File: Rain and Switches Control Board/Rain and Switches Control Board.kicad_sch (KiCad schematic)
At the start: 35 parts, among them J1 Conn_01x06_MountingPin, J2 Screw_Terminal_01x02, J3 Conn_01x02, J4 8P8C, J5 Conn_01x02, J6 Conn_01x02, J7 Conn_01x02, J8 Conn_01x02, J9 RJ45, Q1 NPN, Q2 NPN, Q3 NPN, Q4 NPN, Q5 NPN, U2 OKI-78SR

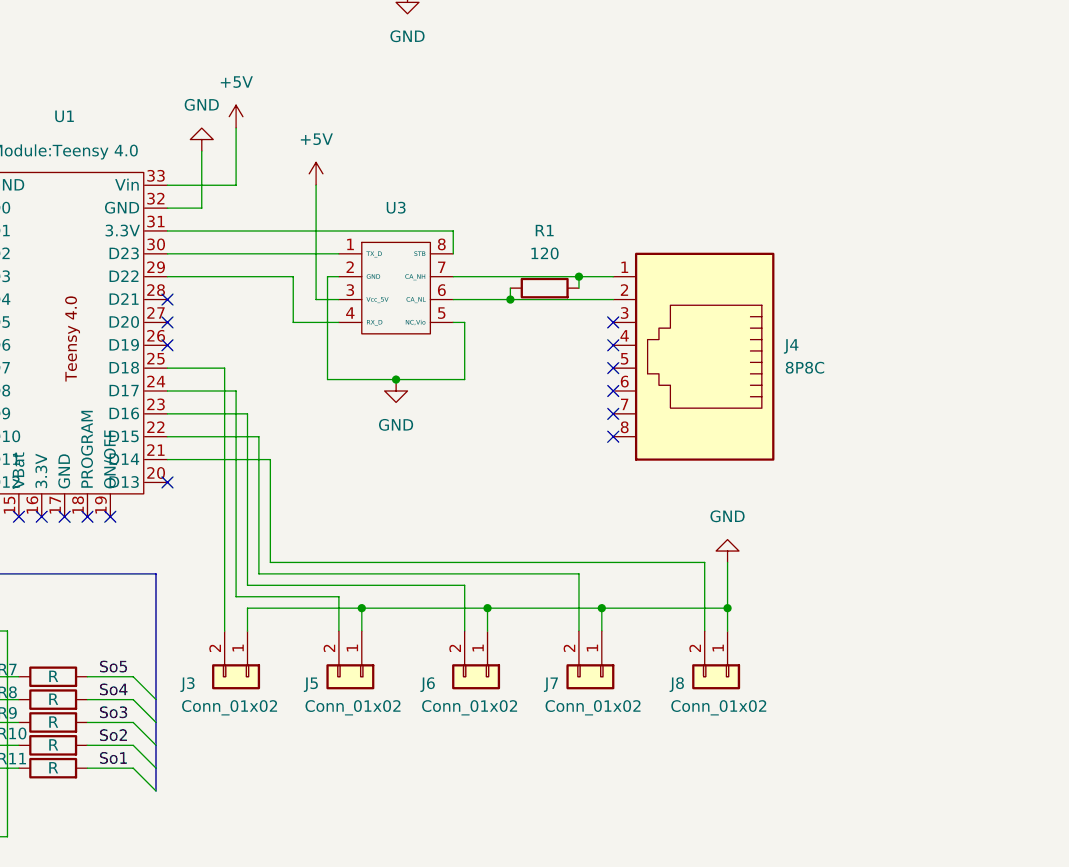
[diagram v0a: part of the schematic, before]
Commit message: Rev. 3
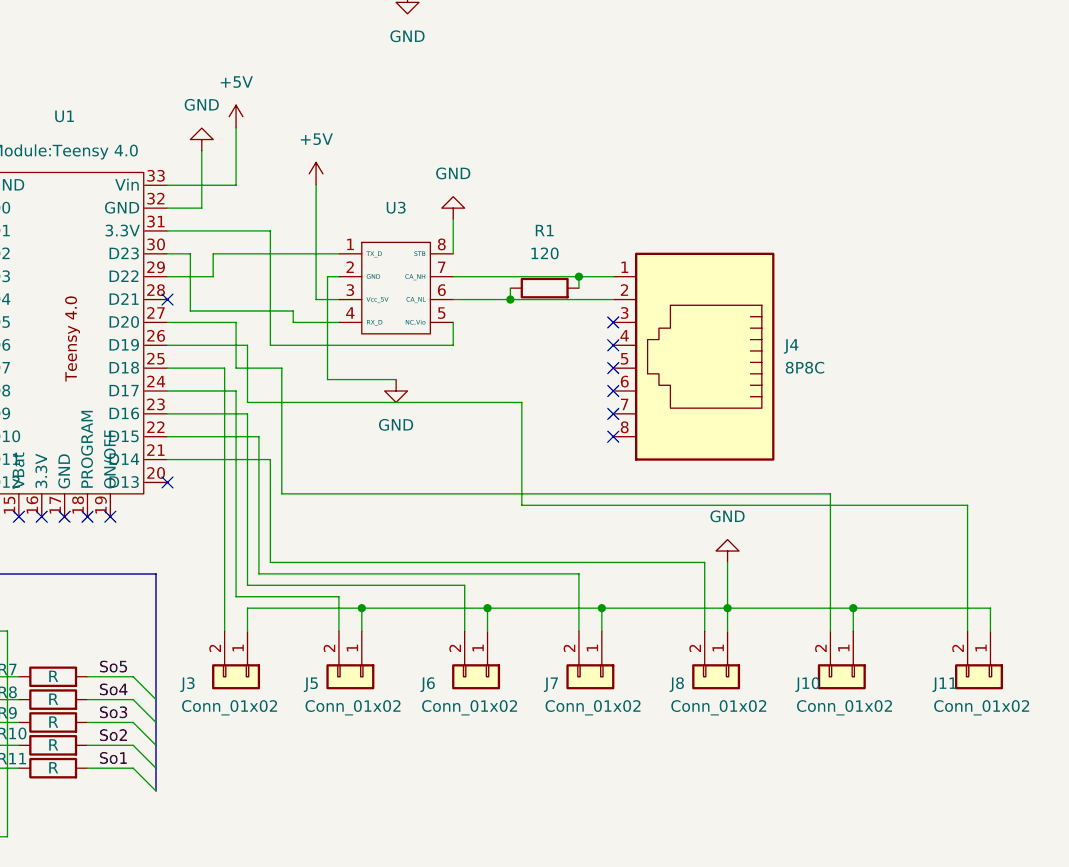
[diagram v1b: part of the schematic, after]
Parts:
- added J10, J11: Conn_01x02, TerminalBlock:TerminalBlock_Altech_AK300-2_P5.00mm, symbol Connector_Generic:Conn_01x02
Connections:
- net GND: now also U3.8 (STB), J10.1 (Pin_1), J11.1 (Pin_1); no longer U3.5 (NC,Vio)
- net at U1.26 (D19): now also J11.2 (Pin_2)
- net at U1.27 (D20): now also J10.2 (Pin_2)
- net at U1.29 (D22): now also U3.1 (TX_D); no longer U3.4 (RX_D)
- net at U1.30 (D23): now also U3.4 (RX_D); no longer U3.1 (TX_D)
- net at U1.31 (3.3V): now also U3.5 (NC,Vio); no longer U3.8 (STB)
- no-connect marks 22 -> 20
